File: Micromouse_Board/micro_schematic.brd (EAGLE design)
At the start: 83.6 x 69.3 mm, 44 parts, among them IC1 L293B, IC2 DSPIC33FJ64MC804-X_PT, J1 61300211121, J2 61300611121, J3 61300311121, J4 61300311121, J5 61300311121, J6 61300611121, U1 TPS62163, U2 Value, Y1 FOXSDLF_160R-20_TR

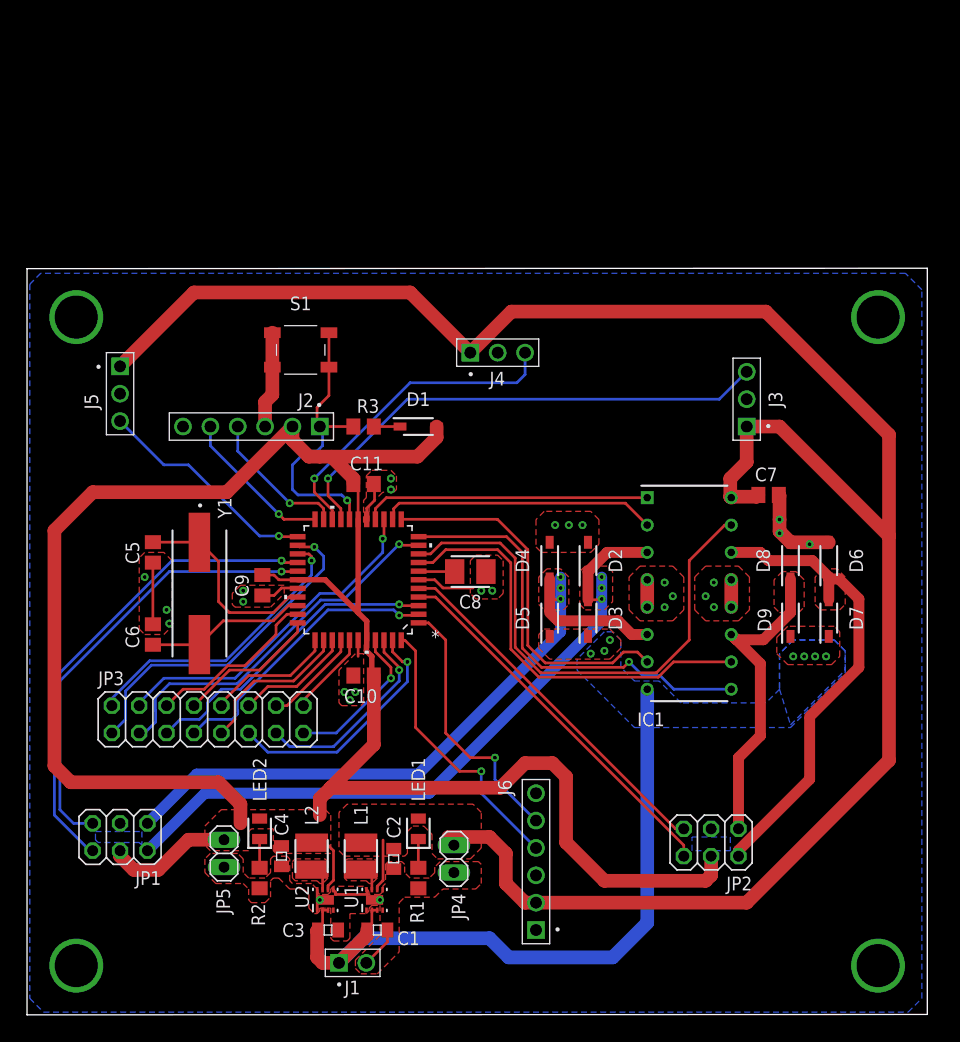
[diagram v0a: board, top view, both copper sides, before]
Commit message: Updated board version
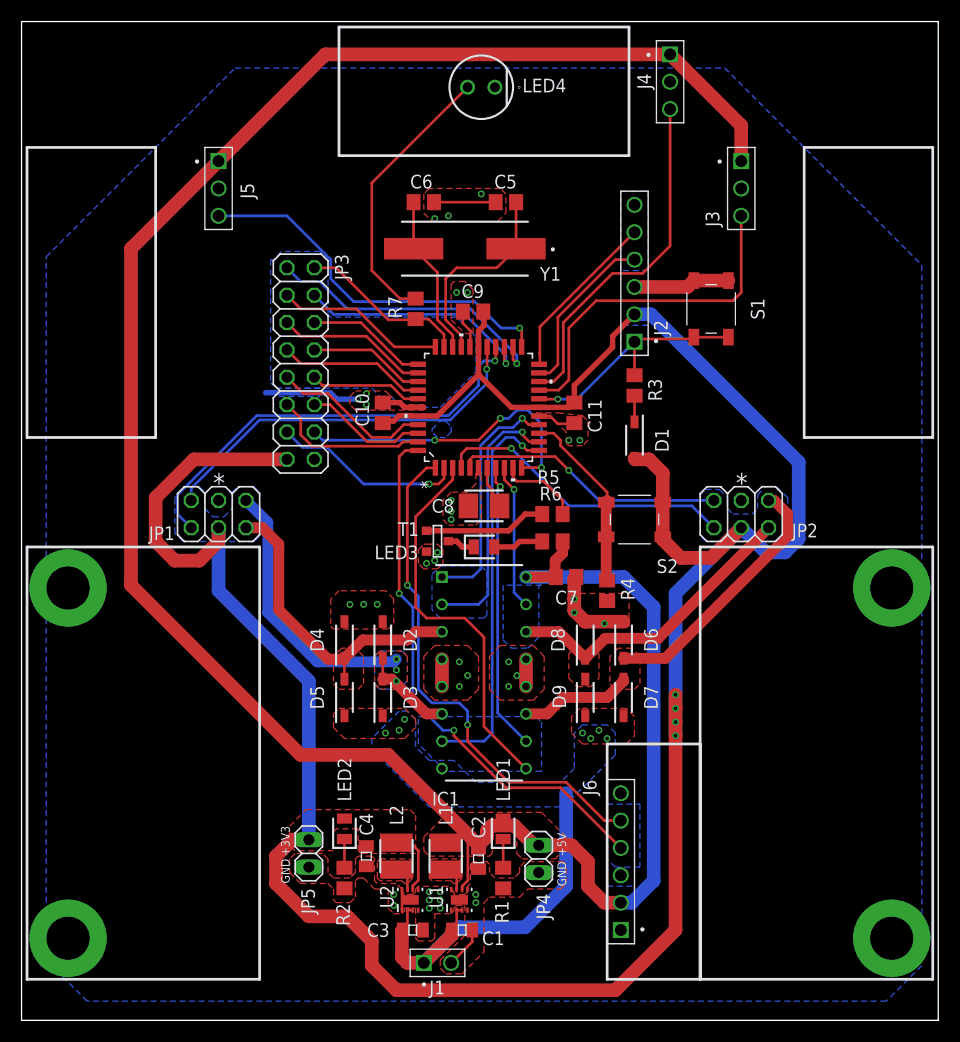
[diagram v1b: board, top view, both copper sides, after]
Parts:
- added LED3: HSME-C170, SamacSys_Parts:LEDC2012X90N
- added LED4: SSL-LX5093TC, SSL-LX5093TC:SSL-LX5093SGC/B
- added R4: 4k7, rcl:R0805
- added R5, R7: 1k, rcl:R0805
- added R6: 180, rcl:R0805
- added S2: PTS647SM50SMTR2LFS, SamacSys_Parts:PTS647SM50SMTR2LFS
- added T1: (no value), zetex:SOT-23
- C5, C6: value 120pF -> 22pF
- U1: value TPS62163 -> Value
- moved C6 47.4 mm to (37.3, 75.9), turned to 0 degrees
- moved C5 46.2 mm to (45.0, 75.9), turned to 180 degrees
- moved Y1 40.4 mm to (41.1, 71.6), turned to 180 degrees
- moved J2 38.3 mm to (56.9, 69.3), turned to 90 degrees
- moved S1 38.3 mm to (64.0, 66.0), turned to 90 degrees
- moved JP3 34.1 mm to (25.9, 61.0), turned to 270 degrees
- moved C9 32.1 mm to (41.9, 65.8), turned to 180 degrees
- moved JP1 31.3 mm to (18.3, 47.0)
- moved JP2 30.6 mm to (66.8, 47.0)
- moved J4 29.8 mm to (60.2, 87.1), turned to 270 degrees
- moved R3 25.4 mm to (56.9, 58.9), turned to 270 degrees
- moved C10 24.4 mm to (33.5, 56.4), turned to 90 degrees
- moved J5 21.1 mm to (18.3, 77.2)
- moved C11 20.6 mm to (51.3, 56.4), turned to 270 degrees
- moved D2 20.4 mm to (33.5, 35.3)
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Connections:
- net N$11 renamed P43
- net N$29 renamed P24
- removed net N$10: IC2.42, JP3.13
- removed net N$12: IC2.38, JP3.16
- removed net N$13: IC2.37, JP3.14
- removed net N$14: IC2.36, JP3.12
- removed net N$15: IC2.35, JP3.9
- removed net N$16: IC2.34, JP3.10
- removed net N$17: IC2.33, JP3.8
- removed net N$18: IC2.32, JP3.6
- removed net N$19: IC2.2, JP3.7
- removed net N$20: IC2.3, JP3.5
- removed net N$23: IC2.10, JP3.3
- removed net N$30: IC2.25, JP3.2
- removed net N$9: IC2.41, JP3.15
- new net BUTTON1: IC2.14, R4.2, S2.3, S2.4
- new net LED3: IC2.10, R5.2
- new net LED4: IC2.32, JP3.2, R7.1
- new net N$21: LED4.2, R7.2
- new net N$6: R5.1, T1.3
- new net N$8: LED3.2, R6.2
- new net P11: IC2.11, JP3.14
- new net P2: IC2.2, JP3.13
- new net P25: IC2.25, JP3.4
- new net P33: IC2.33, JP3.3
- new net P34: IC2.34, JP3.6
- new net P35: IC2.35, JP3.5
- new net P36: IC2.36, JP3.8
- new net P37: IC2.37, JP3.7
- new net P38: IC2.38, JP3.10
- new net P41: IC2.41, JP3.9
- new net P42: IC2.42, JP3.12
- net +3V3: now also JP3.15, S2.1, S2.2
- net +5V: now also R6.1
- net GND: now also JP3.16, LED4.1, R4.1, T1.2
- net M1_1: now also D4.1, D5.2; no longer D2.1, D3.2
- net M1_2: now also D2.1, D3.2; no longer D4.1, D5.2
- net M2_1: now also D8.1, D9.2; no longer D6.1, D7.2
- net M2_2: now also D6.1, D7.2; no longer D8.1, D9.2
- net N$22: now also LED3.1, T1.1; no longer IC2.14, JP3.4
- net PWM2: now also IC2.3; no longer IC2.11
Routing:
- net +3V3: track 196.7 -> 249.8 mm, vias 0 -> 4
- net M1_1: track 74.2 -> 29.8 mm, vias 3 -> 0
- net ME2_1: track 49.3 -> 13.5 mm, vias 0 -> 1
- net N$23: track 34.6 -> 0.00 mm, vias 1 -> 0
- net M1_2: track 67.7 -> 34.0 mm
- net N$22: track 31.8 -> 2.59 mm, vias 1 -> 0
- net P11: track 0.00 -> 29.0 mm, vias 0 -> 3
- net N$20: track 28.8 -> 0.00 mm, vias 1 -> 0
- net VBAT: track 70.2 -> 41.9 mm
- net N$30: track 27.0 -> 0.00 mm, vias 1 -> 0
- net N$19: track 26.6 -> 0.00 mm, vias 1 -> 0
- net N$21: track 0.00 -> 25.8 mm
- net TX_B: track 25.9 -> 50.4 mm, vias 1 -> 2
- net RX_B: track 24.7 -> 48.0 mm, vias 1 -> 2
- net P25: track 0.00 -> 22.5 mm, vias 0 -> 1
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- added copper zone on layer 16, net M1_2
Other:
- board size 83.6 x 69.3 mm -> 85.1 x 92.7 mm
- board text added: "*"
- board text added: "+3V3"
- board text added: "+5V"
- board text added: "GND"
